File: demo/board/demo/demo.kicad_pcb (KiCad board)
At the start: 2 copper layers, 25 parts, among them J2 Conn_01x20, J3 Conn_01x20, J6 FTSH-107-01-F-DV-K, U1 STM32F413CGUx, U2 LD1117S33TR_SOT223, U4 MAX33054EASA+T, Y1 CSTNE8M00

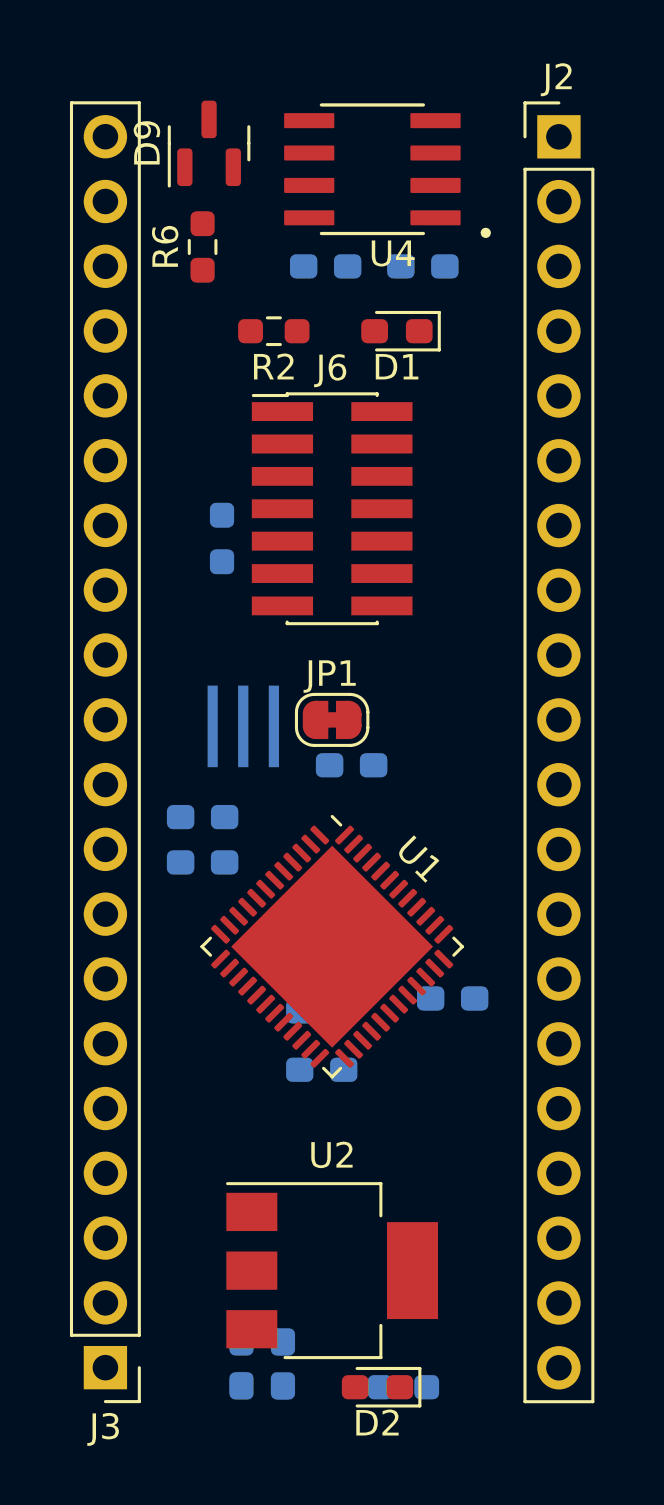
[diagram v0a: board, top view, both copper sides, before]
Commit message: finished demo board schem and layout
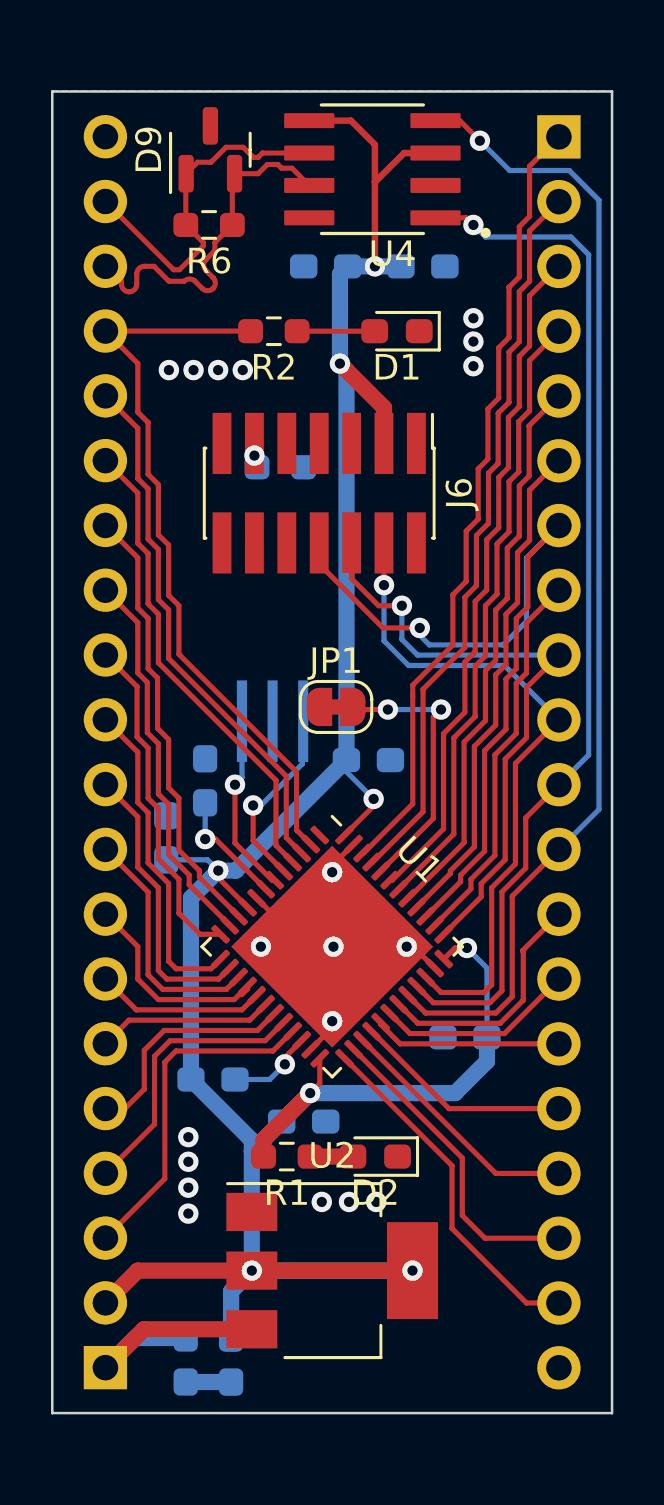
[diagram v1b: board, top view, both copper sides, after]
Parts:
- J2, J3: moved to B.Cu
- R1: moved to F.Cu
- moved R1 10.1 mm to (151.9, 99.7), turned to 180 degrees
- moved D2 9.04 mm to (155.4, 99.7)
- moved C7 4.38 mm to (152.6, 98.3), turned to 0 degrees
- moved C4 4.28 mm to (149.0, 96.6), turned to 180 degrees
- moved R10 3.61 mm to (151.6, 72.6), turned to 180 degrees
- moved C2 2.19 mm to (147.9, 107.6)
- moved C3 2.04 mm to (149.7, 107.6)
- moved C9 1.72 mm to (147.2, 87.2), turned to 90 degrees
- moved C11 1.60 mm to (158.9, 95.0)
- moved C5 1.43 mm to (148.7, 84.9), turned to 90 degrees
- moved Y1 1.17 mm to (151.3, 82.6)
- moved R6 0.90 mm to (148.8, 63.1), turned to 180 degrees
- moved J6 0.79 mm to (153.2, 73.7), turned to -90 degrees
- moved C10 0.69 mm to (155.1, 84.1)
- moved JP1 0.53 mm to (153.8, 82.0)
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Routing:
- net +3V3: track 0.00 -> 111.2 mm, vias 0 -> 8
- net A11: track 0.00 -> 45.0 mm, vias 0 -> 1
- net A12: track 0.00 -> 40.7 mm, vias 0 -> 1
- net B3_TRACESWO: track 0.00 -> 32.6 mm, vias 0 -> 1
- net B9: track 0.00 -> 31.3 mm
- net C13: track 0.00 -> 29.1 mm
- net B8: track 0.00 -> 29.0 mm
- net B7: track 0.00 -> 26.9 mm
- net A13_SWDIO: track 0.00 -> 26.4 mm, vias 0 -> 1
- net B6: track 0.00 -> 24.5 mm
- net A14_SWCLK: track 0.00 -> 24.4 mm, vias 0 -> 1
- net B5: track 0.00 -> 22.2 mm
- net C14: track 0.00 -> 21.1 mm
- net B4: track 0.00 -> 19.8 mm
- net C15: track 0.00 -> 18.8 mm
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- added copper zone on B.Cu, net GND
- added copper zone on F.Cu, net GND
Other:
- board outline added: 21.9 x 51.8 mm
